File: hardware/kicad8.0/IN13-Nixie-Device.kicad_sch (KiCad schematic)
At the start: 40 parts, among them J1 PINHD_1x3_Female, J2 AudioJack3, J3 PINHD_1x4_Male, J4 USB_C_Receptacle_USB2.0_16P, J5 PINHD_1x4_Male, Q2 MMBTA42, SW1 SW_Push, SW3 SW_Push, T1 Transformer_1P_1S, U1 LM358, U2 STI3508, U3 AMS1117-3.3, U4 ESP32-C6-MINI-1/U

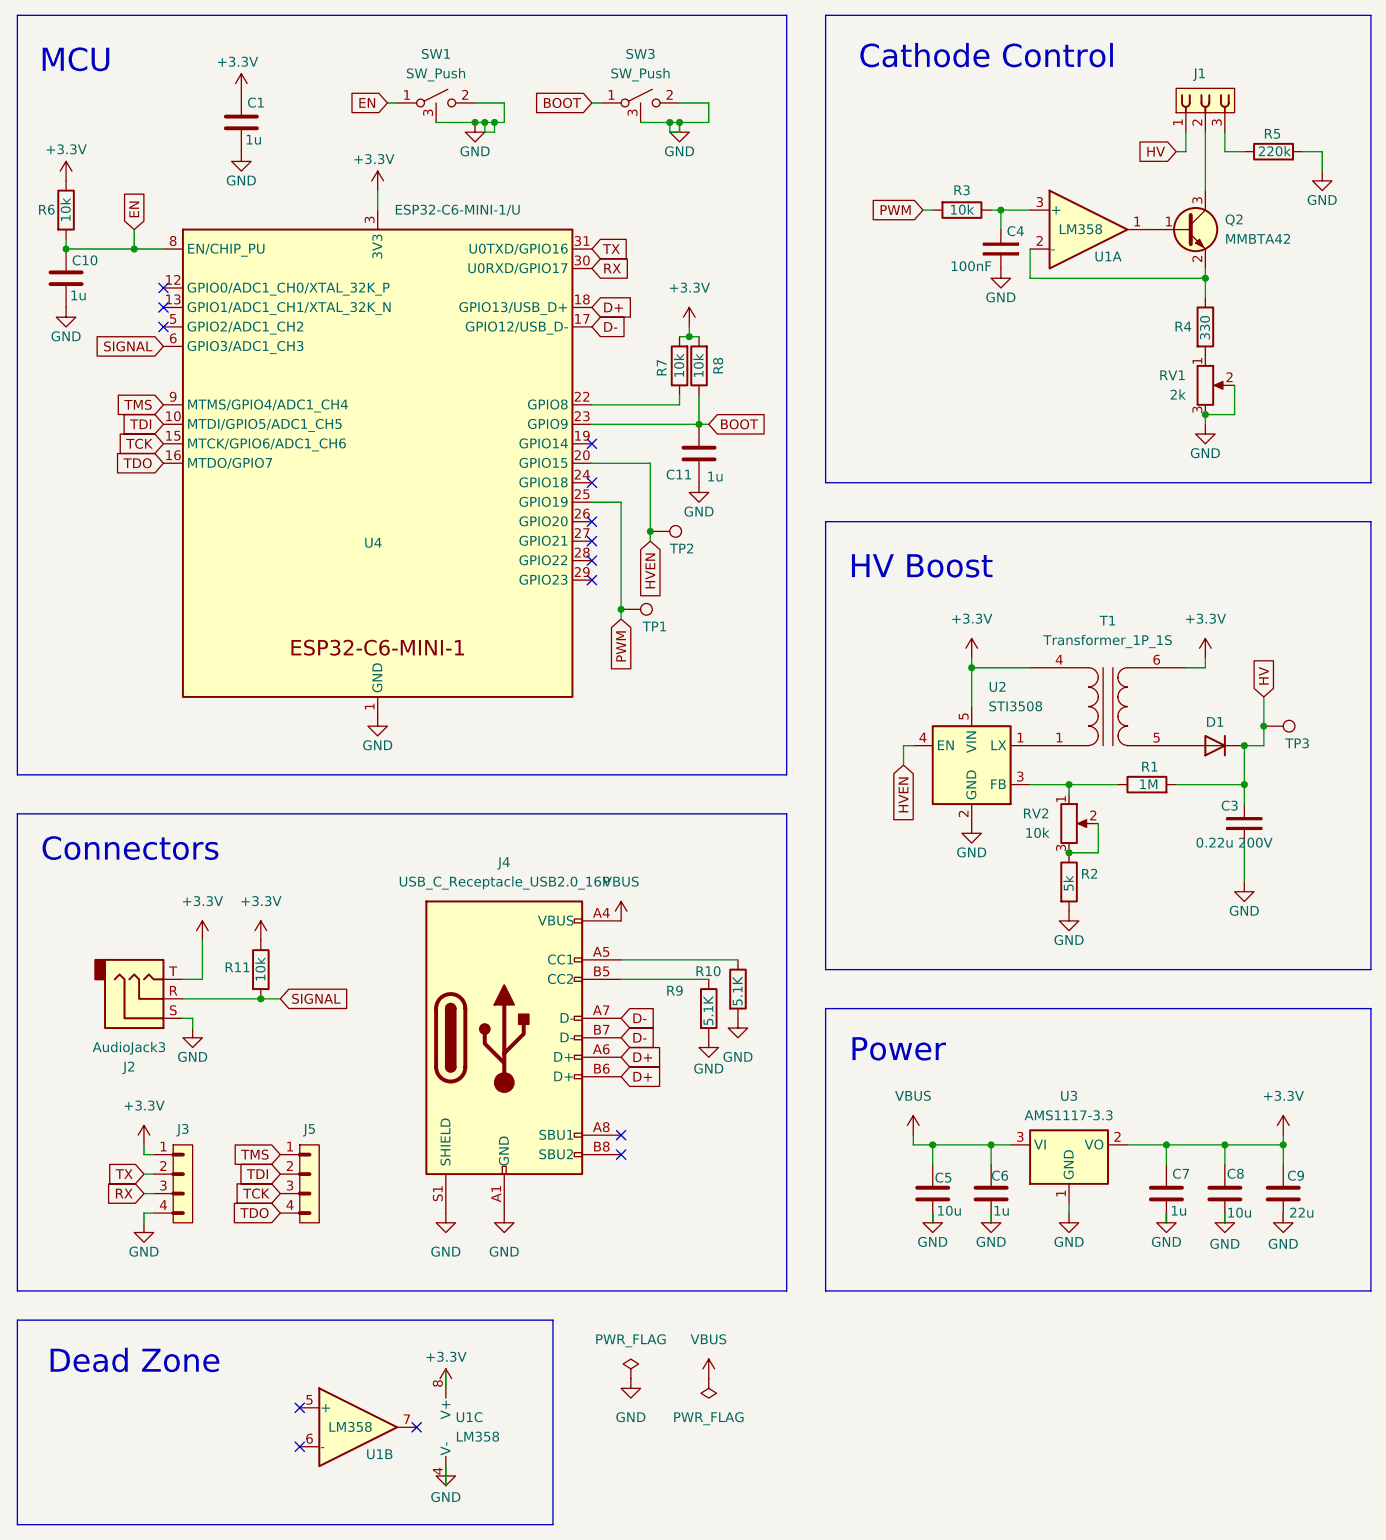
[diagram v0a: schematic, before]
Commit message: pcb revision
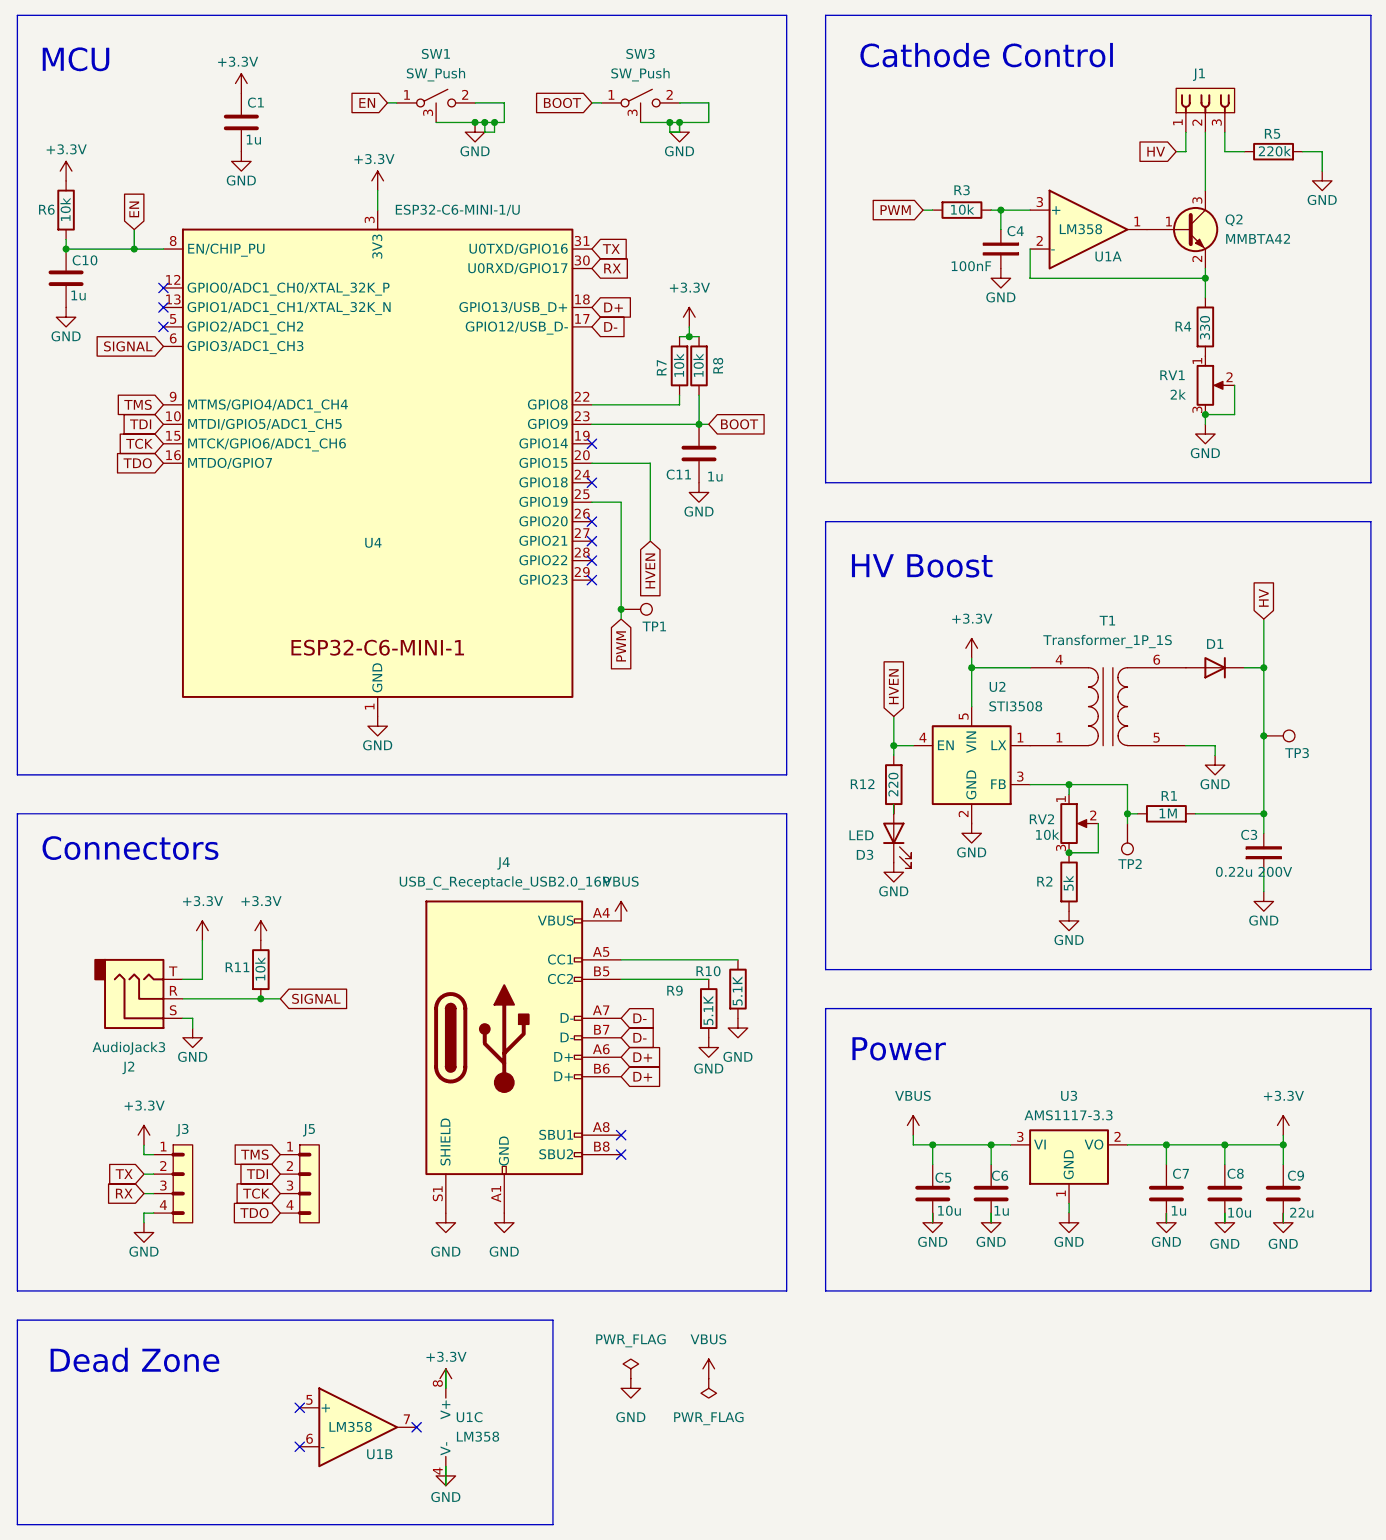
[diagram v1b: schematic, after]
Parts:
- added D3: LED, LED_SMD:LED_0603_1608Metric, symbol Device:LED
- added R12: 220, Resistor_SMD:R_0603_1608Metric, symbol Device:R
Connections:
- net +3.3V: no longer T1.6 (SB)
- net GND: now also T1.5 (SA), D3.1 (K)
- net HVEN: now also R12.2; no longer TP2.1
- net at D1.2 (A): now also T1.6 (SB); no longer T1.5 (SA)
- net at R1.1, RV2.1, U2.3 (FB): now also TP2.1
- new net: D3.2 (A), R12.1
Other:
- moved on the sheet: C3, D1, R1, TP3
